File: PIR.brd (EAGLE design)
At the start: 20.3 x 25.1 mm, 3 parts, among them X1 IR

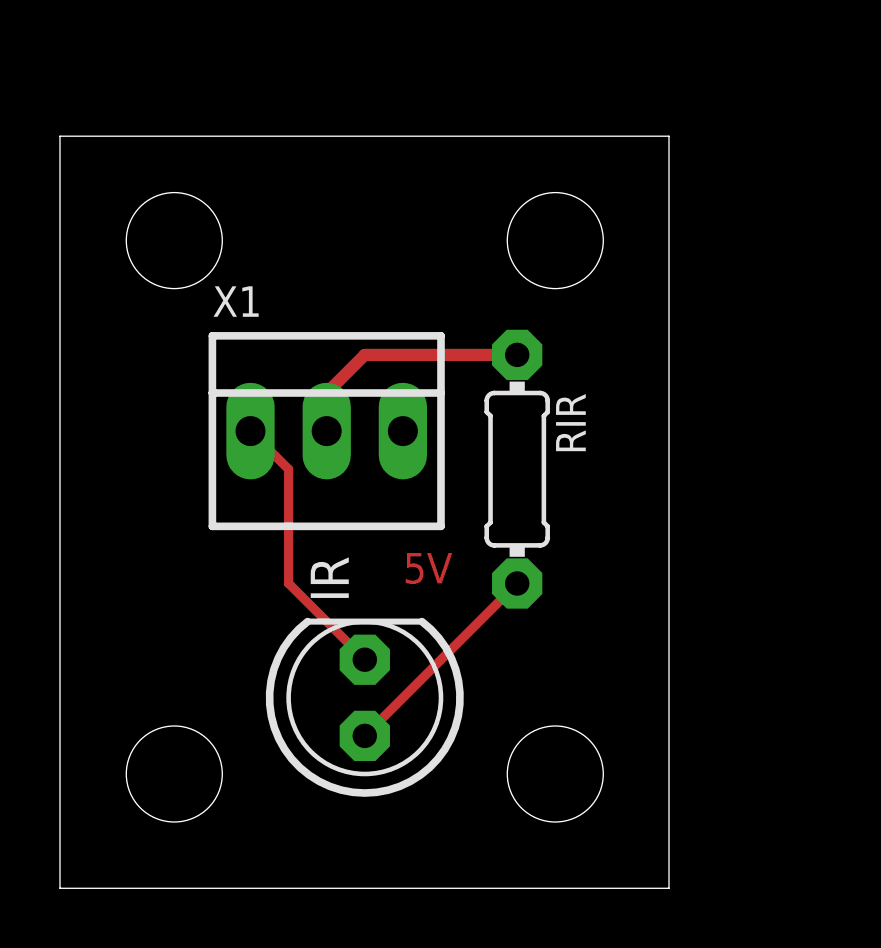
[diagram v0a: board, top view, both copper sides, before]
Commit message: 29/10/2013
Fixed:
-Naming in PIN
-PIR & Light Sensor PCB
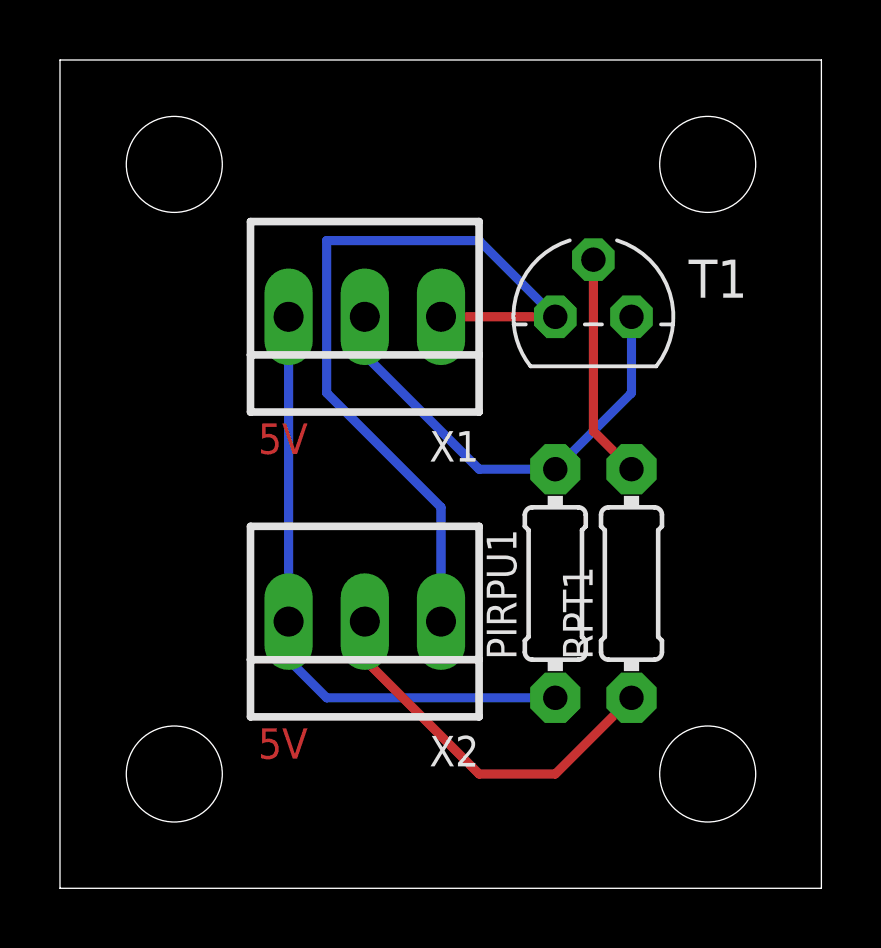
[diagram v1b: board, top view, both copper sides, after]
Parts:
- removed IR: (no value), adafruit:LED5MM
- removed RIR: 220, adafruit:0204/7
- added PIRPU1: 10K, adafruit:0204/7
- added RPT1: 4K7, adafruit:0204/7
- added T1: 2N3904, transistor-neu-to92:TO92
- added X2: PIR, con-molex:22-23-2031
- X1: value IR -> SIGNAL
- moved X1 4.02 mm to (10.2, 19.1), turned to 180 degrees
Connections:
- removed net N$2: RIR.1, X1.2
- removed net N$4: IR.A, RIR.2
- new net N$10: RPT1.1, X2.2
- new net N$12: RPT1.2, T1.2
- new net SIG: PIRPU1.2, T1.1, X1.2
- net +5V: now also PIRPU1.1, X2.3
- net GND: now also T1.3, X2.1; no longer IR.K
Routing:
- net +5V: track 0.00 -> 20.8 mm
- net GND: track 9.20 -> 26.8 mm
- net SIG: track 0.00 -> 15.3 mm
- net N$10: track 0.00 -> 12.8 mm
- net N$2: track 8.15 -> 0.00 mm
- net N$12: track 0.00 -> 7.51 mm
- net N$4: track 7.18 -> 0.00 mm
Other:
- board size 20.3 x 25.1 mm -> 25.4 x 27.6 mm
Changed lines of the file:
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@@
 <setting verticaltext="up"/>
 </settings>
-<grid distance="0.05" unitdist="inch" unit="inch" style="lines" multiple="1" display="yes" altdistance="0.025" altunitdist="inch" altunit="inch"/>
+<grid distance="0.02" unitdist="inch" unit="inch" style="lines" multiple="1" display="yes" altdistance="0.025" altunitdist="inch" altunit="inch"/>
 <layers>
 <layer number="1" name="Top" color="4" fill="1" visible="yes" active="yes"/>
@@
 <board>
 <plain>
-<wire x1="0" y1="0" x2="20.3" y2="0" width="0" layer="20"/>
-<wire x1="20.3" y1="0" x2="20.3" y2="25.07" width="0" layer="20"/>
-<wire x1="20.3" y1="25.07" x2="0" y2="25.07" width="0" layer="20"/>
-<wire x1="0" y1="25.07" x2="0" y2="0" width="0" layer="20"/>
-<hole x="16.51" y="3.81" drill="3.2"/>
+<wire x1="0" y1="0" x2="25.38" y2="0" width="0" layer="20"/>
+<wire x1="25.38" y1="0" x2="25.38" y2="27.61" width="0" layer="20"/>
+<wire x1="25.38" y1="27.61" x2="0" y2="27.61" width="0" layer="20"/>
+<wire x1="0" y1="27.61" x2="0" y2="0" width="0" layer="20"/>
+<hole x="21.59" y="3.81" drill="3.2"/>
 <hole x="3.81" y="3.81" drill="3.2"/>
-<hole x="3.81" y="21.59" drill="3.2"/>
-<hole x="16.51" y="21.59" drill="3.2"/>
-<text x="11.43" y="10.16" size="1.016" layer="1">5V</text>
+<hole x="21.59" y="24.13" drill="3.2"/>
+<hole x="3.81" y="24.13" drill="3.2"/>
+<text x="6.604" y="14.478" size="1.016" layer="1">5V</text>
+<text x="6.604" y="4.318" size="1.016" layer="1">5V</text>
 </plain>
 <attributes>
@@
 </variantdefs>
 <classes>
-<class number="0" name="default" width="0" drill="0">
+<class number="0" name="default" width="0.254" drill="0">
+<clearance class="0" value="0.254"/>
 </class>
 </classes>
@@
 <param name="RoutingGrid" value="50mil"/>
 <param name="tpViaShape" value="round"/>
-<param name="PrefDir.1" value="|"/>
+<param name="PrefDir.1" value="*"/>
 <param name="PrefDir.2" value="0"/>
 <param name="PrefDir.3" value="0"/>
@@
 <param name="PrefDir.14" value="0"/>
 <param name="PrefDir.15" value="0"/>
-<param name="PrefDir.16" value="0"/>
+<param name="PrefDir.16" value="*"/>
 <param name="cfVia" value="8"/>
 <param name="cfNonPref" value="5"/>
@@
 </autorouter>
 <elements>
-<element name="X1" library="con-molex" package="22-23-2031" value="IR" x="8.89" y="15.24">
-<attribute name="OC_NEWARK" value="30C0862" x="26.67" y="8.89" size="1.778" layer="27" display="off"/>
-<attribute name="MPN" value="22-23-2031" x="26.67" y="8.89" size="1.778" layer="27" display="off"/>
-<attribute name="MF" value="MOLEX" x="26.67" y="8.89" size="1.778" layer="27" display="off"/>
-<attribute name="OC_FARNELL" value="1462950" x="26.67" y="8.89" size="1.778" layer="27" display="off"/>
+<element name="RPT1" library="adafruit" package="0204/7" value="4K7" x="19.05" y="10.16" rot="R90"/>
+<element name="PIRPU1" library="adafruit" package="0204/7" value="10K" x="16.51" y="10.16" rot="R90"/>
+<element name="X1" library="con-molex" package="22-23-2031" value="SIGNAL" x="10.16" y="19.05" rot="R180">
+<attribute name="OC_NEWARK" value="30C0862" x="-7.62" y="25.4" size="1.778" layer="27" rot="R180" display="off"/>
+<attribute name="MPN" value="22-23-2031" x="-7.62" y="25.4" size="1.778" layer="27" rot="R180" display="off"/>
+<attribute name="MF" value="MOLEX" x="-7.62" y="25.4" size="1.778" layer="27" rot="R180" display="off"/>
+<attribute name="OC_FARNELL" value="1462950" x="-7.62" y="25.4" size="1.778" layer="27" rot="R180" display="off"/>
 </element>
-<element name="RIR" library="adafruit" package="0204/7" value="220" x="15.24" y="13.97" rot="R270"/>
-<element name="IR" library="adafruit" package="LED5MM" value="" x="10.16" y="6.35" rot="R90"/>
+<element name="X2" library="con-molex" package="22-23-2031" value="PIR" x="10.16" y="8.89" rot="R180">
+<attribute name="OC_NEWARK" value="30C0862" x="-16.51" y="15.24" size="1.778" layer="27" rot="R180" display="off"/>
+<attribute name="MPN" value="22-23-2031" x="-16.51" y="15.24" size="1.778" layer="27" rot="R180" display="off"/>
+<attribute name="MF" value="MOLEX" x="-16.51" y="15.24" size="1.778" layer="27" rot="R180" display="off"/>
+<attribute name="OC_FARNELL" value="1462950" x="-16.51" y="15.24" size="1.778" layer="27" rot="R180" display="off"/>
+</element>
+<element name="T1" library="transistor-neu-to92" package="TO92" value="2N3904" x="17.78" y="19.05"/>
 </elements>
 <signals>
-<signal name="N$2">
+<signal name="GND">
+<contactref element="X2" pad="1"/>
+<contactref element="T1" pad="3"/>
+<contactref element="X1" pad="1"/>
+<wire x1="12.7" y1="19.05" x2="16.51" y2="19.05" width="0.3048" layer="1"/>
+<wire x1="12.7" y1="12.7" x2="12.7" y2="8.89" width="0.3048" layer="16"/>
+<wire x1="8.89" y1="16.51" x2="12.7" y2="12.7" width="0.3048" layer="16"/>
+<wire x1="8.89" y1="21.59" x2="8.89" y2="16.51" width="0.3048" layer="16"/>
+<wire x1="13.97" y1="21.59" x2="8.89" y2="21.59" width="0.3048" layer="16"/>
+<wire x1="16.51" y1="19.05" x2="13.97" y2="21.59" width="0.3048" layer="16"/>
+</signal>
+<signal name="+5V">
+<contactref element="PIRPU1" pad="1"/>
+<contactref element="X2" pad="3"/>
+<contactref element="X1" pad="3"/>
+<wire x1="7.62" y1="19.05" x2="7.62" y2="8.89" width="0.3048" layer="16"/>
+<wire x1="8.89" y1="6.35" x2="16.51" y2="6.35" width="0.3048" layer="16"/>
+<wire x1="7.62" y1="7.62" x2="8.89" y2="6.35" width="0.3048" layer="16"/>
+<wire x1="7.62" y1="8.89" x2="7.62" y2="7.62" width="0.3048" layer="16"/>
+</signal>
+<signal name="N$10">
+<contactref element="RPT1" pad="1"/>
+<contactref element="X2" pad="2"/>
+<wire x1="10.16" y1="7.62" x2="10.16" y2="8.89" width="0.3048" layer="1"/>
+<wire x1="13.97" y1="3.81" x2="10.16" y2="7.62" width="0.3048" layer="1"/>
+<wire x1="16.51" y1="3.81" x2="13.97" y2="3.81" width="0.3048" layer="1"/>
+<wire x1="19.05" y1="6.35" x2="16.51" y2="3.81" width="0.3048" layer="1"/>
+</signal>
+<signal name="N$12">
+<contactref element="RPT1" pad="2"/>
+<contactref element="T1" pad="2"/>
+<wire x1="17.78" y1="15.24" x2="17.78" y2="20.955" width="0.3048" layer="1"/>
+<wire x1="19.05" y1="13.97" x2="17.78" y2="15.24" width="0.3048" layer="1"/>
+</signal>
+<signal name="SIG">
 <contactref element="X1" pad="2"/>
-<contactref element="RIR" pad="1"/>
-<wire x1="8.89" y1="15.24" x2="8.89" y2="16.51" width="0.4064" layer="1"/>
-<wire x1="8.89" y1="16.51" x2="10.16" y2="17.78" width="0.4064" layer="1"/>
-<wire x1="10.16" y1="17.78" x2="15.24" y2="17.78" width="0.4064" layer="1"/>
-</signal>
-<signal name="N$4">
-<contactref element="RIR" pad="2"/>
-<contactref element="IR" pad="A"/>
-<wire x1="15.24" y1="10.16" x2="10.16" y2="5.08" width="0.3048" layer="1"/>
-</signal>
-<signal name="GND">
-<contactref element="X1" pad="1"/>
-<contactref element="IR" pad="K"/>
-<wire x1="7.62" y1="13.97" x2="6.35" y2="15.24" width="0.3048" layer="1"/>
-<wire x1="7.62" y1="10.16" x2="7.62" y2="13.97" width="0.3048" layer="1"/>
-<wire x1="10.16" y1="7.62" x2="7.62" y2="10.16" width="0.3048" layer="1"/>
-</signal>
-<signal name="+5V">
-<contactref element="X1" pad="3"/>
+<contactref element="PIRPU1" pad="2"/>
+<contactref element="T1" pad="1"/>
+<wire x1="19.05" y1="16.51" x2="19.05" y2="19.05" width="0.3048" layer="16"/>
+<wire x1="16.51" y1="13.97" x2="19.05" y2="16.51" width="0.3048" layer="16"/>
+<wire x1="10.16" y1="17.78" x2="10.16" y2="19.05" width="0.3048" layer="16"/>
+<wire x1="13.97" y1="13.97" x2="10.16" y2="17.78" width="0.3048" layer="16"/>
+<wire x1="16.51" y1="13.97" x2="13.97" y2="13.97" width="0.3048" layer="16"/>
 </signal>
 </signals>
